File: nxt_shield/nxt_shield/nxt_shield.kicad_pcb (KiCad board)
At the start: 2 copper layers, 125.6 x 62.8 mm, 77 parts, among them J1 NXT_M0, J10 NXT_SENS0, J11 NXT_SENS0, J12 NXT_SENS0, J13 JST_RB_I2C1, J14 JST_RB_I2C2, J15 JST_RB_I2C3, J16 JST_RB_I2C4, J17 RB_I2C1, J18 RB_I2C0, J19 RB_I2C2, J2 RB_M0, J20 RB_I2C3, J21 RB_I2C4, J22 RB_I2C5, J23 RB_I2C6, J24 RB_I2C7, J25 RB_Power, J26 JST_RB_I2C5, J27 JST_RB_I2C6, J28 JST_RB_I2C7, J3 NXT_SENS0, J4 RB_M0, J5 NXT_M1, J6 RB_M0, J7 NXT_M2, J8 LCD, J9 JST_RB_I2C0, U1 74HC14, U3 TPS4H000

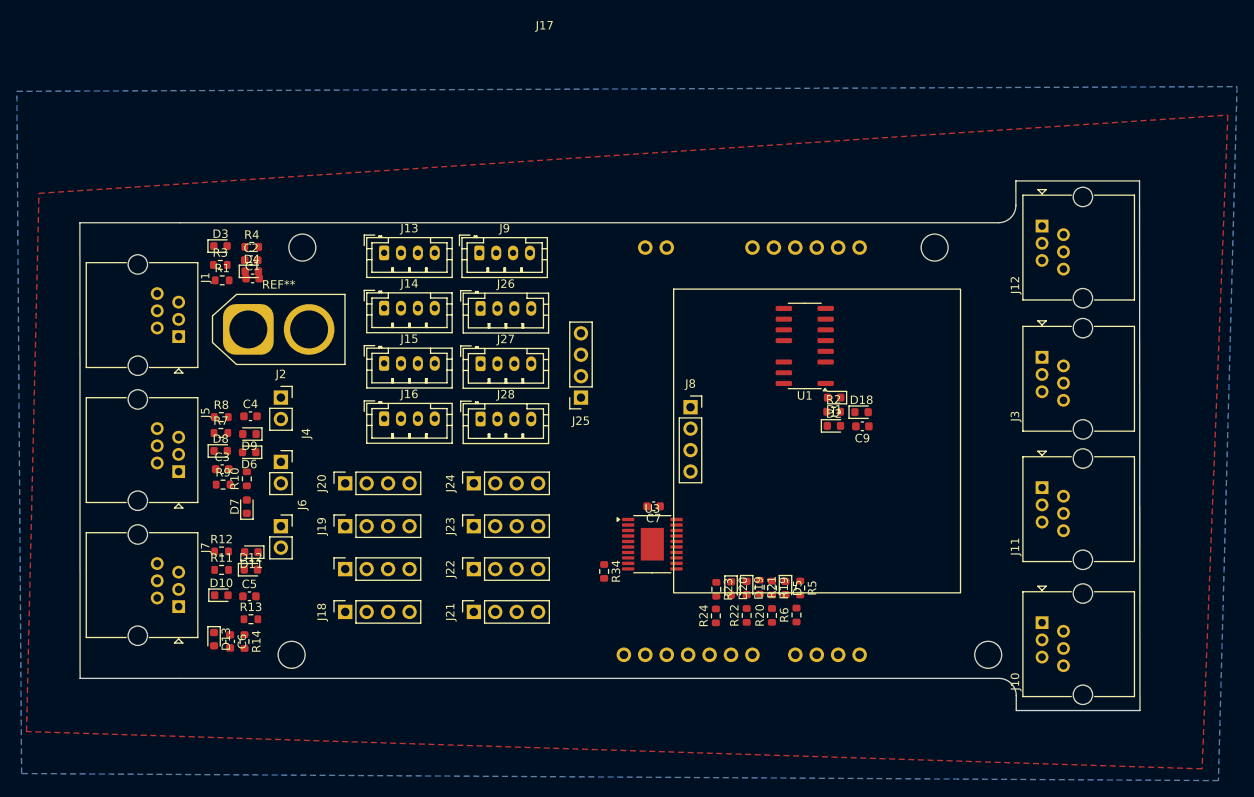
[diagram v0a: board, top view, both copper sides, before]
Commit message: nxt shield first prototype production
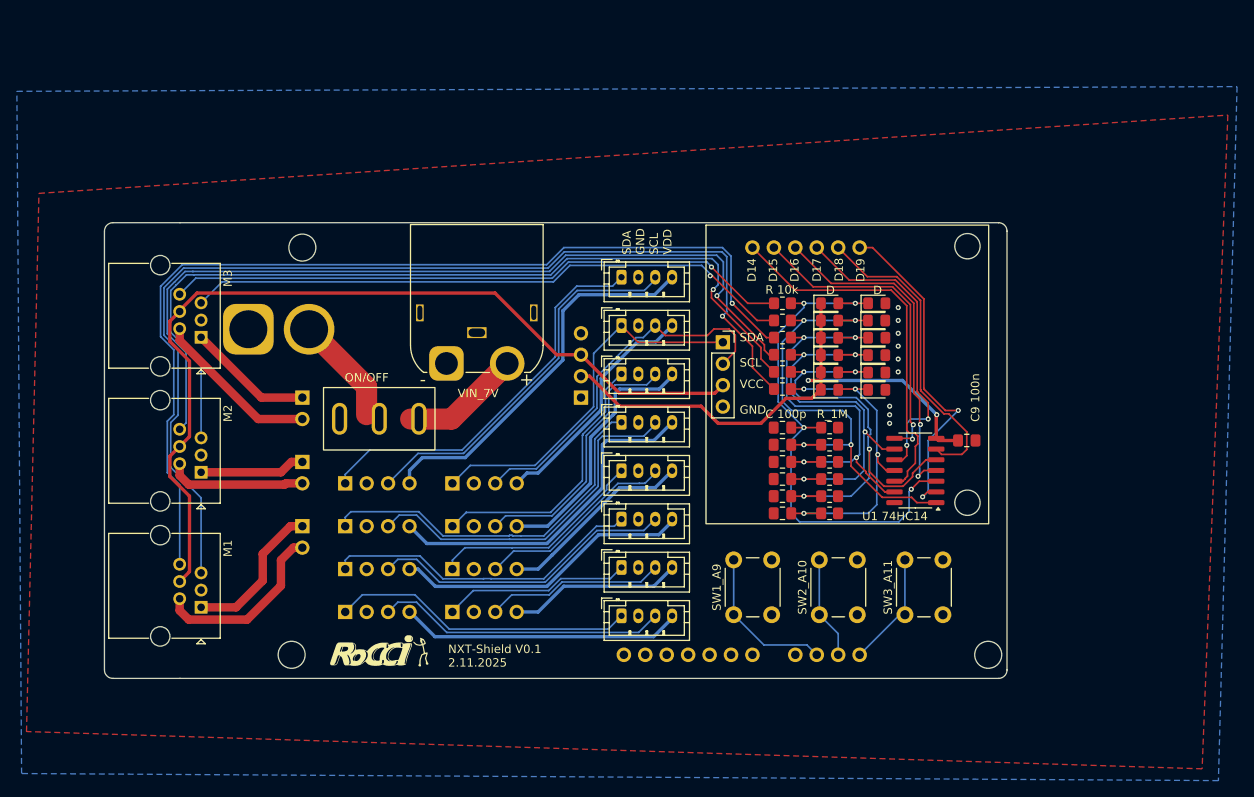
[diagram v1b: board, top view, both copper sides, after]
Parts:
- removed C7: 100n, Capacitor_SMD:C_0603_1608Metric
- removed D18, D19, D20, D5: D, Diode_SMD:D_0603_1608Metric
- removed J11, J12: NXT_SENS0, Connector_RJ:RJ25_Wayconn_MJEA-660X1_Horizontal
- removed R19, R20, R21, R22, R23, R24, R5, R6: 1k, Resistor_SMD:R_0603_1608Metric
- removed R34: 820, Resistor_SMD:R_0603_1608Metric
- removed REF**: AMASS_XT60-M_1x02_P7.20mm_Vertical, Connector_AMASS:AMASS_XT60-M_1x02_P7.20mm_Vertical
- removed U3: TPS4H000, Package_SO:HTSSOP-20-1EP_4.4x6.5mm_P0.65mm_EP2.74x3.86mm
- added G***: LOGO, external_libs:RocciLogo, F.Cu at (116.6, 106.2)
- added G***: LOGO, external_libs:RocciLogo, B.Cu at (132.3, 106.7)
- added ON/OFF: SW_SPDT, CustomFootprints:XKB Connection SS-12M11G5, F.Cu at (115.1, 76.4)
- added SW1_A9: SW_Push, Button_Switch_THT:SW_PUSH_6mm, F.Cu at (158.6, 101.9)
- added SW2_A10: SW_Push, Button_Switch_THT:SW_PUSH_6mm, F.Cu at (168.7, 101.9)
- added SW3_A11: SW_Push, Button_Switch_THT:SW_PUSH_6mm, F.Cu at (178.9, 101.9)
- C1, C2, C3, C4, C5, C6: footprint Capacitor_SMD:C_0603_1608Metric -> Capacitor_SMD:C_0805_2012Metric_Pad1.18x1.45mm_HandSolder
- C9 100n: renamed from C9; footprint Capacitor_SMD:C_0603_1608Metric -> Capacitor_SMD:C_0805_2012Metric_Pad1.18x1.45mm_HandSolder
- D1, D10, D11, D12, D13, D2, D3, D4, D6, D7, D8, D9: footprint Diode_SMD:D_0603_1608Metric -> Diode_SMD:D_0805_2012Metric_Pad1.15x1.40mm_HandSolder
- J17, J18, J19, J20, J21, J22, J23, J24, J25: moved to B.Cu
- J3: value NXT_SENS0 -> XT60_PCB; footprint Connector_RJ:RJ25_Wayconn_MJEA-660X1_Horizontal -> Connector_AMASS:AMASS_XT60-M_1x02_P7.20mm_Vertical; moved to B.Cu
- J4: value RB_M0 -> RB_M2; moved to B.Cu
- J6: value RB_M0 -> RB_M1; moved to B.Cu
- J8: footprint Connector_PinSocket_2.54mm:PinSocket_1x04_P2.54mm_Vertical -> CustomFootprints:OLE_LCD
- R1, R10, R11, R12, R13, R14, R2, R3, R4, R7, R8, R9: footprint Resistor_SMD:R_0603_1608Metric -> Resistor_SMD:R_0805_2012Metric_Pad1.20x1.40mm_HandSolder
- RB 7V: renamed from J2; value RB_M0 -> RB_M3; moved to B.Cu
- U1 74HC14: renamed from U1; footprint Package_SO:SOIC-14-16_3.9x9.9mm_P1.27mm -> Package_SO:SO-14_3.9x8.65mm_P1.27mm
- VIN_7V: renamed from J10; value NXT_SENS0 -> XT60_Case; footprint Connector_RJ:RJ25_Wayconn_MJEA-660X1_Horizontal -> Connector_AMASS:AMASS_XT60IPW-M_1x03_P7.20mm_Horizontal
- moved J3 94.1 mm to (101.0, 68.1), turned to 0 degrees
- moved D13 86.3 mm to (175.5, 69.1), turned to 0 degrees
- moved D8 78.3 mm to (175.5, 73.2)
- moved D12 77.2 mm to (175.5, 75.3)
- moved VIN_7V 77.0 mm to (124.5, 72.2), turned to 0 degrees
- moved D10 76.1 mm to (169.9, 75.3)
- moved D9 74.9 mm to (175.5, 71.2), turned to 0 degrees
- moved D4 74.2 mm to (175.5, 65.0)
- moved D11 73.1 mm to (169.9, 69.1), turned to 0 degrees
- moved R14 72.5 mm to (169.9, 83.8), turned to 0 degrees
- moved D3 72.5 mm to (169.9, 65.0)
- moved R9 71.9 mm to (169.9, 87.9)
- moved R4 71.7 mm to (169.9, 79.8)
- moved D7 71.4 mm to (169.9, 71.2), turned to 0 degrees
- moved R12 71.1 mm to (164.3, 69.1)
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- renumbered J7 to M1, J5 to M2, J1 to M3
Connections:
- net Net-(J1-Pin_1) renamed /M0A
- net Net-(J1-Pin_2) renamed /M0B
- net Net-(J4-Pin_1) renamed /M1A
- net Net-(J4-Pin_2) renamed /M1B
- net Net-(J6-Pin_1) renamed /M2A
- net Net-(J6-Pin_2) renamed /M2B
- A1 pad A1: SENS_P4 -> (no net)
- A1 pad A10: SENS_DIAG0 -> Button2
- A1 pad A11: THERMAL_0 -> Button3
- A1 pad A2: SENS_P3 -> (no net)
- A1 pad A3: SENS_P2 -> (no net)
- A1 pad A4: SENS_P1 -> (no net)
- A1 pad A5: SENS3_ADC -> unconnected-(A1-PadA5)
- A1 pad A6: SENS2_ADC -> unconnected-(A1-PadA6)
- A1 pad A7: SENS1_ADC -> unconnected-(A1-PadA7)
- A1 pad A8: SENS0_ADC -> unconnected-(A1-PadA8)
- A1 pad A9: SENS_DIAG1 -> Button1
- J13 pad 4: +3.3V -> VDDI2C1
- J14 pad 4: +3.3V -> VDDI2C2
- J15 pad 4: +3.3V -> VDDI2C3
- J16 pad 4: +3.3V -> VDDI2C4
- J17 pad 4: +3.3V -> VDDI2C1
- J18 pad 4: +3.3V -> VDDI2C0
- J19 pad 4: +3.3V -> VDDI2C2
- J20 pad 4: +3.3V -> VDDI2C3
- J21 pad 4: +3.3V -> VDDI2C4
- J22 pad 4: +3.3V -> VDDI2C5
- J23 pad 4: +3.3V -> VDDI2C6
- J24 pad 4: +3.3V -> VDDI2C7
- J26 pad 4: +3.3V -> VDDI2C5
- J27 pad 4: +3.3V -> VDDI2C6
- J28 pad 4: +3.3V -> VDDI2C7
- J3 pad 1: SENS0_9V -> GND
- J3 pad 2: GND -> /AKKU1
- J8 pad 3: GND -> +5V
- J8 pad 4: +5V -> GND
- J9 pad 4: +3.3V -> VDDI2C0
- VIN_7V pad 1: SENS1_9V -> GND
- VIN_7V pad 2: GND -> /AKKU2
- VIN_7V pad 3: GND -> (no net)
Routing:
- net ENC_M2_A: track 0.00 -> 123.5 mm, vias 0 -> 1
- net ENC_M2_B: track 0.00 -> 116.7 mm, vias 0 -> 1
- net +5V: track 0.00 -> 106.5 mm
- net ENC_M1_A: track 0.00 -> 101.8 mm, vias 0 -> 1
- net ENC_M1_B: track 0.00 -> 100.2 mm, vias 0 -> 1
- net ENC_M0_B: track 0.00 -> 74.1 mm, vias 0 -> 1
- net ENC_M0_A: track 0.00 -> 72.6 mm, vias 0 -> 1
- net +3.3V: track 0.00 -> 66.5 mm, vias 0 -> 2
- net Net-(D3-A): track 0.00 -> 63.8 mm, vias 0 -> 4
- net Net-(D1-A): track 0.00 -> 57.4 mm, vias 0 -> 4
- net Net-(D6-A): track 0.00 -> 57.0 mm, vias 0 -> 4
- net Net-(D11-A): track 0.00 -> 50.7 mm, vias 0 -> 4
- net Net-(D7-A): track 0.00 -> 48.5 mm, vias 0 -> 4
- net SDA3: track 0.00 -> 46.9 mm
- net VDDI2C3: track 0.00 -> 45.5 mm
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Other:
- board size 125.6 x 62.8 mm -> 107 x 54 mm
- board text added: "C 100p"
- board text added: "D"
- board text added: "D14"
- board text added: "D15"
- board text added: "D16"
- board text added: "D17"
- board text added: "D18"
- board text added: "D19"
- board text added: "NXT-Shield V0.1 2.11.2025"
- board text added: "R 10k"
- board text added: "R_1M"
- board text added: "SDA GND SCL VDD"
